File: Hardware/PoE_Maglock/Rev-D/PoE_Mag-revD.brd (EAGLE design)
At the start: 91.8 x 45.4 mm, 90 parts, among them IC2 ATMEGA32U4-MU, J2 1X2-3.5MM, J3 1X2-3.5MM, J4 1X2-3.5MM, J5 1X2-3.5MM, J6 10103594-0001LF, Q1 35A/25V/8.5mΩ, Q3 35A/25V/8.5mΩ, Q5 35A/25V/8.5mΩ, Q6 35A/25V/8.5mΩ, SW1 SPST_TACT-KMR2, T1 DMG3415U, U2 SPX3819-3.3, U3 LMV358IDGKR, U4 W5500, X2 J1011FHANRUN, Y4 8MHz

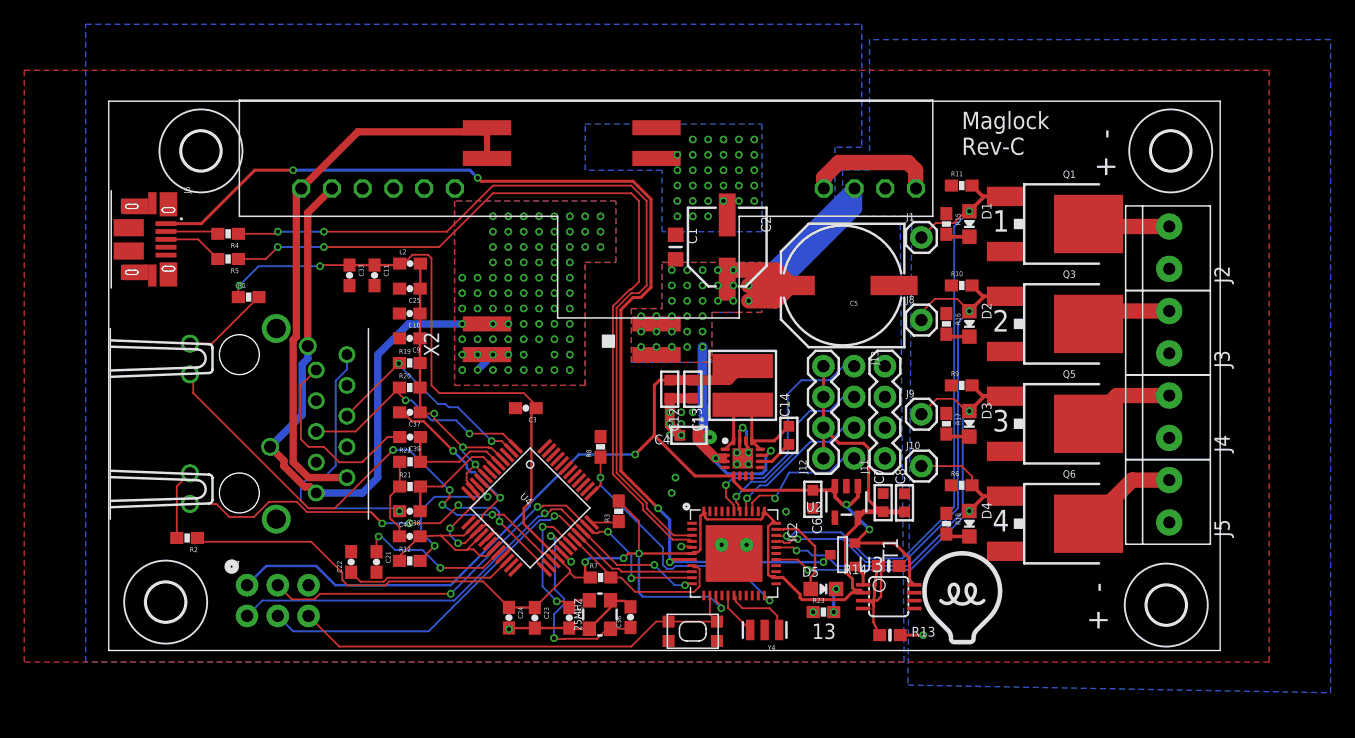
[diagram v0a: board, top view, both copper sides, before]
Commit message: HEEP-654 passive poe maglock for review
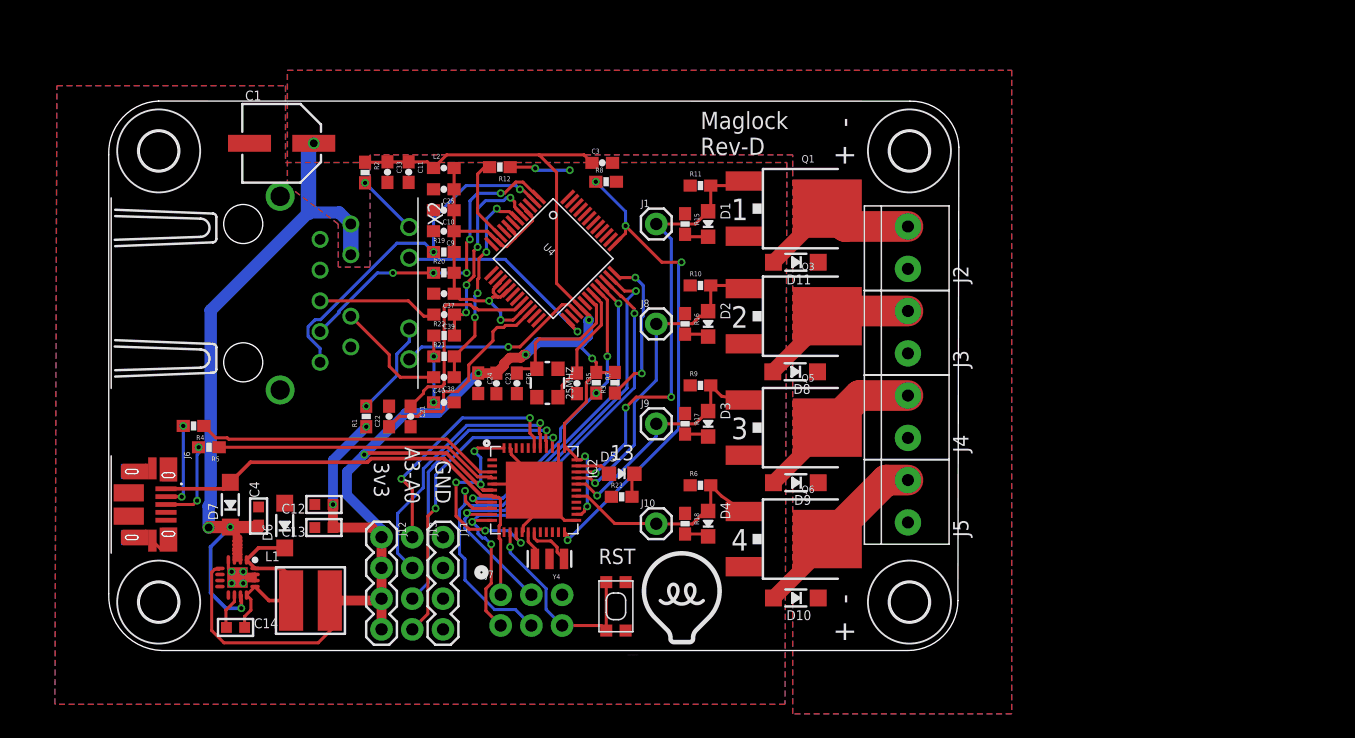
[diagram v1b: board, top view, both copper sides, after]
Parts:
- removed C2: 100uF 25V, microbuilder:PANASONIC_D
- removed C5: 470uF 25V, SparkFun-Passives:PANASONIC_G
- removed C6, C8: 10µF, microbuilder:0603-MINI
- removed C7: 1uF, microbuilder:0603-MINI
- removed R13, R14: 10K, microbuilder:0603-NO
- removed T1: DMG3415U, zetex:SOT-23
- removed U$1: SILVERTEL_POEMICRO, Heep:AG9900
- removed U$16: AG5200AG5300, Heep:AG5300
- removed U2: SPX3819-3.3, microbuilder:SOT23-5
- removed U3: LMV358IDGKR, linear:MSOP08
- added D10, D11, D8, D9: (no value), microbuilder:SOD-123
- added D6, D7: PMEG4030ER, microbuilder:SOD-123
- C1: value 10uF -> (none); device microbuilder:_0805MP -> microbuilder:PANASONIC_D
- X2: value J1011FHANRUN -> J1011FTOP_TAB; device Heep:HANRUN_POE -> Heep:HANRUN_HR971169C
- moved C14 48.4 mm to (11.1, 2.22), turned to 0 degrees
- moved U$19 42.9 mm to (11.3, 6.35), turned to 270 degrees
- moved L1 39.9 mm to (17.3, 4.45), turned to 0 degrees
- moved J13 39.2 mm to (25.7, 9.68)
- moved J12 37.1 mm to (23.2, 9.68), turned to 270 degrees
- moved J11 37.1 mm to (28.3, 9.68), turned to 270 degrees
- moved C4 36.2 mm to (13.0, 11.4), turned to 90 degrees
- moved C1 33.7 mm to (14.9, 42.2), turned to 0 degrees
- moved R2 33.6 mm to (21.8, 39.8), turned to 270 degrees
- moved R12 33.4 mm to (33.0, 40.3), turned to 180 degrees
- moved C13 32.6 mm to (18.4, 10.5), turned to 180 degrees
- moved C12 30.1 mm to (18.4, 12.4), turned to 180 degrees
- moved U$15 23.2 mm to (43.5, 0.00)
- moved J10 22.4 mm to (45.9, 10.8)
- moved J1 21.9 mm to (45.9, 35.6)
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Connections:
- removed net +5V: C12.1, C13.1, C6.1, J7.2, L1.P$2, T1.2, U$19.P5, U2.1, U2.3, U3.8
- removed net CMP: R13.1, R14.2, U3.3
- removed net GATE_CMD: T1.3, U3.1
- removed net N$1: U$1.VIN-1, U$1.VIN-2, U$16.P$2, X2.10
- removed net N$15: C14.2, L1.P$1, U$19.P1, U$19.P12, U$19.P13, U$19.P16
- removed net N$2: U$1.VIN+1, U$1.VIN+2, U$16.P$1, X2.9
- new net N$16: C14.2, D6.C, L1.P$1, U$19.P1, U$19.P12, U$19.P13, U$19.P16
- net +3V3: now also C12.1, C13.1, L1.P$2, U$19.P5; no longer C7.1, C8.1, U2.5, U3.2
- net ACTLED: now also X2.P11; no longer X2.12
- net DRAIN1: now also D11.A
- net DRAIN2: now also D8.A
- net DRAIN3: now also D9.A
- net DRAIN4: now also D10.A
- net GND: now also C1.-, D6.A, X2.M2, X2.P7, X2.P9; no longer C1.1, C2.-, C5.-, C6.2, C7.2, C8.2, R14.1, U$1.V-, U$16.P$10, U$16.P$7, U2.2, U3.4
- net LNKLED: now also X2.P13; no longer X2.14
- net N$3: now also X2.P14; no longer X2.13
- net N$4: now also X2.P12; no longer X2.11
- net RD+: now also X2.P4; no longer X2.1
- net RD-: now also X2.P5; no longer X2.2
- net TDN: now also X2.P3; no longer X2.6
- net TDP: now also X2.P1; no longer X2.5
- net VBAT: now also C1.+, D10.C, D11.C, D7.C, D8.C, D9.C, X2.P10, X2.P8; no longer C1.2, C2.+, C5.+, R13.2, U$1.V+1, U$1.V+2, U$16.P$8
- net VBUS: now also D7.A, J7.2; no longer T1.1
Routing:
- net +5V: track 86.4 -> 0.00 mm, vias 3 -> 0
- net N$1: track 57.0 -> 0.00 mm, vias 86 -> 0
- net VBUS: track 91.4 -> 38.0 mm, vias 5 -> 0
- net N$2: track 47.8 -> 0.00 mm
- net D+: track 68.3 -> 23.6 mm, vias 2 -> 0
- net D-: track 68.4 -> 25.4 mm, vias 2 -> 0
- net GND: track 67.1 -> 32.6 mm, vias 55 -> 6
- net ACTLED: track 42.6 -> 15.9 mm, vias 4 -> 1
- net RST: track 38.0 -> 17.3 mm, vias 0 -> 1
- net EN2: track 44.8 -> 26.7 mm, vias 2 -> 1
- net LNKLED: track 35.7 -> 17.7 mm, vias 4 -> 1
- net EN3: track 37.9 -> 20.1 mm, vias 2 -> 1
- net N$16: track 0.00 -> 17.3 mm
- net WIZ_RST: track 23.5 -> 40.4 mm, vias 2 -> 4
- net EN1: track 52.3 -> 36.8 mm, vias 2 -> 3
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- removed copper zone on layer 1, net N$1
- removed copper zone on layer 16, net N$1
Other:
- board size 91.8 x 45.4 mm -> 70.2 x 45.4 mm
- board text added: "3v3"
- board text added: "A3-A0"
- board text added: "GND"
- board text added: "Maglock Rev-D"
- board text added: "RST"
- board text removed: "Maglock Rev-C"

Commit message: HEEP-688 updated value
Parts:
- C1: value (none) -> 100uF 25V
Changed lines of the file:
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@@
 <element name="D6" library="microbuilder" package="SOD-123" value="PMEG4030ER" x="15.176853125" y="10.643746875" rot="R90"/>
 <element name="D7" library="microbuilder" package="SOD-123" value="PMEG4030ER" x="10.682984375" y="12.3671" rot="R90"/>
-<element name="C1" library="microbuilder" package="PANASONIC_D" value="" x="14.9225" y="42.2275"/>
+<element name="C1" library="microbuilder" package="PANASONIC_D" value="100uF 25V" x="14.9225" y="42.2275"/>
 <element name="D8" library="microbuilder" package="SOD-123" value="" x="57.353796875" y="23.35" rot="R180"/>
 <element name="D9" library="microbuilder" package="SOD-123" value="" x="57.4125" y="14.1831125" rot="R180"/>
